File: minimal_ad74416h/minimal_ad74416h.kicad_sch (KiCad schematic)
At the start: 82 parts, among them U2 AD74416HBCPZ-RL7, U3 ADR4525BRZ

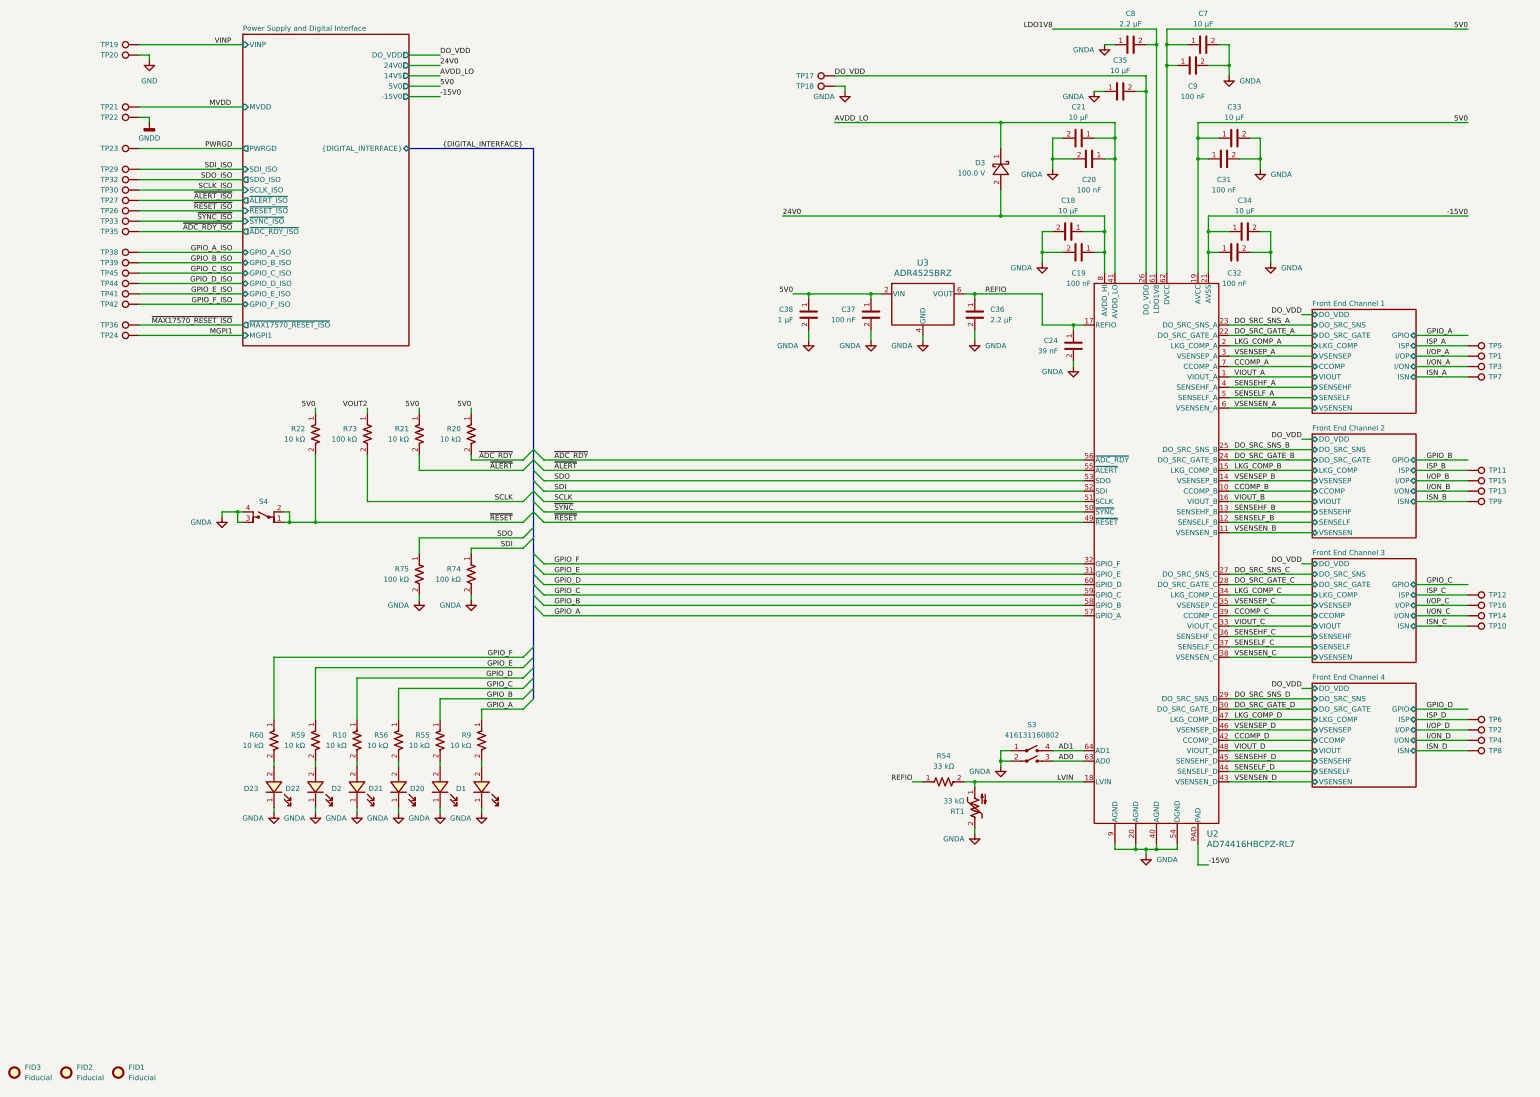
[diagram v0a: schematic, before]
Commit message: backup
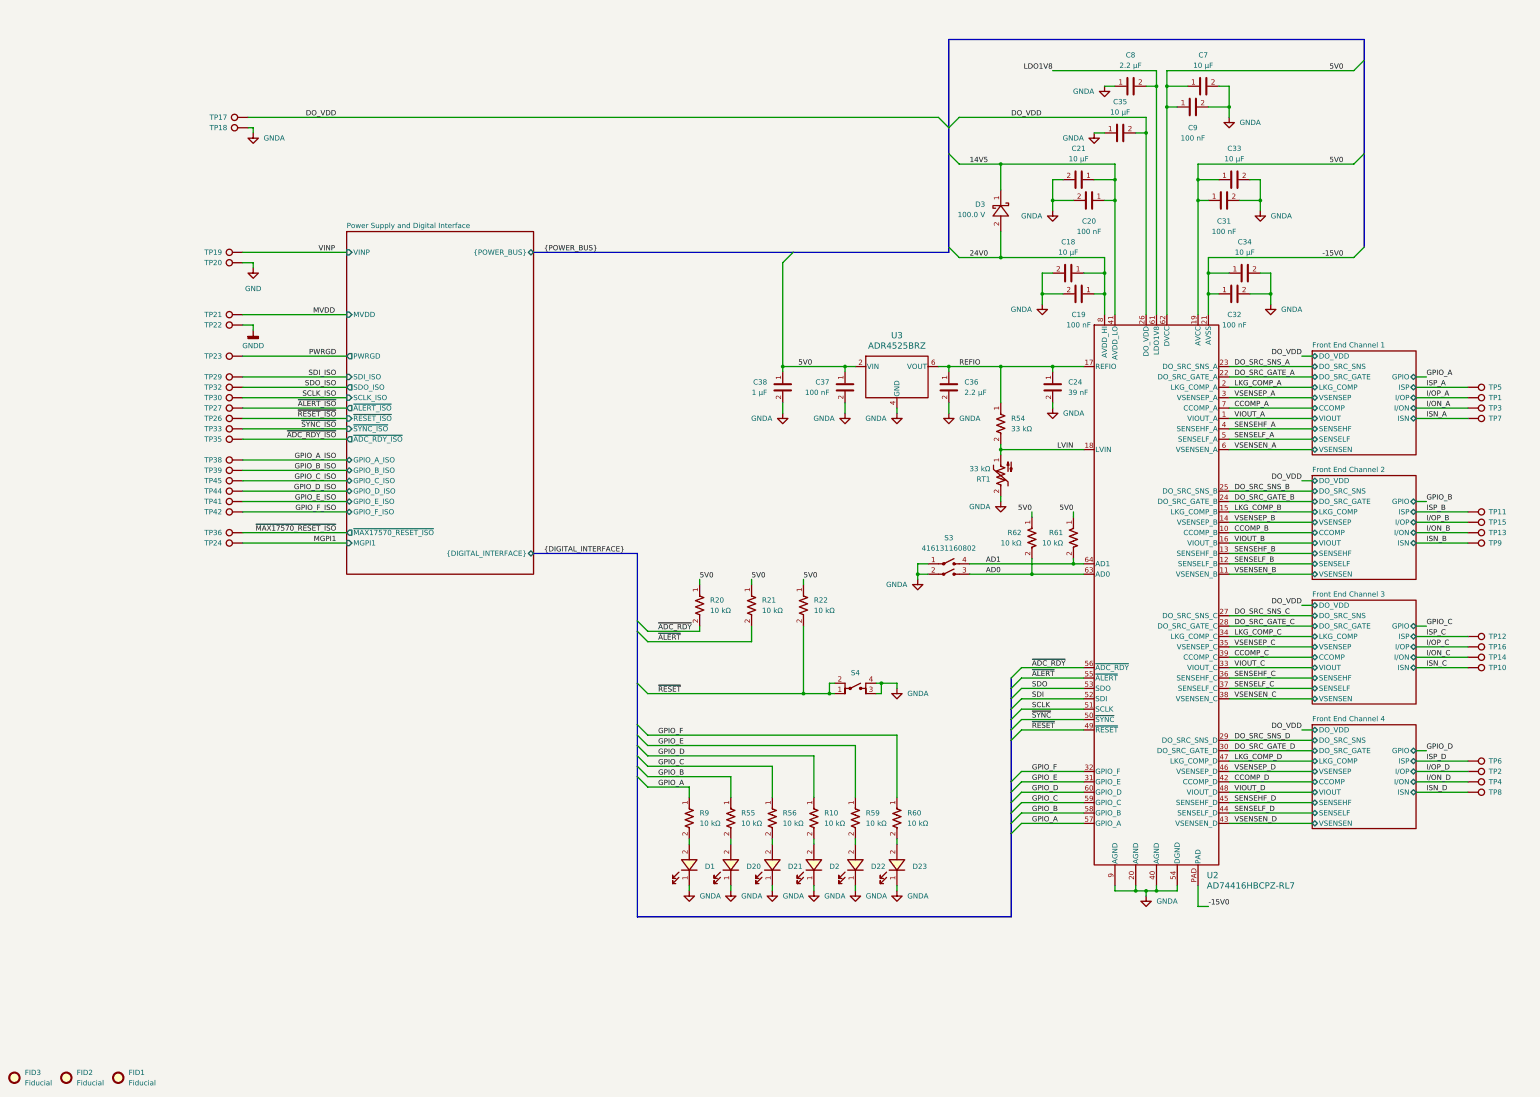
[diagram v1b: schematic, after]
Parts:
- removed R73, R74, R75: 100 kΩ, resistor_footprints:R_0402_1005Metric, symbol UNITED_RESISTORS_DATA_BASE:R_ERJ-2GEJ104X
- added R61, R62: 10 kΩ, resistor_footprints:R_0402_1005Metric, symbol UNITED_RESISTORS_DATA_BASE:R_ERJ-2RKF1002X
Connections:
- net 5V0: now also R61.1, R62.1
- net AD0: now also R62.2
- net AD1: now also R61.2
- net AVDD_LO renamed 14V5
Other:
- sheet Power Supply and Digital Interface ports: added {POWER_BUS}; removed -15V0, 14V5, 24V0, 5V0, DO_VDD
- moved on the sheet: C18, C19, C20, C21, C24, C31, C32, C33, C34, C35, C36, C37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

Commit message: backup
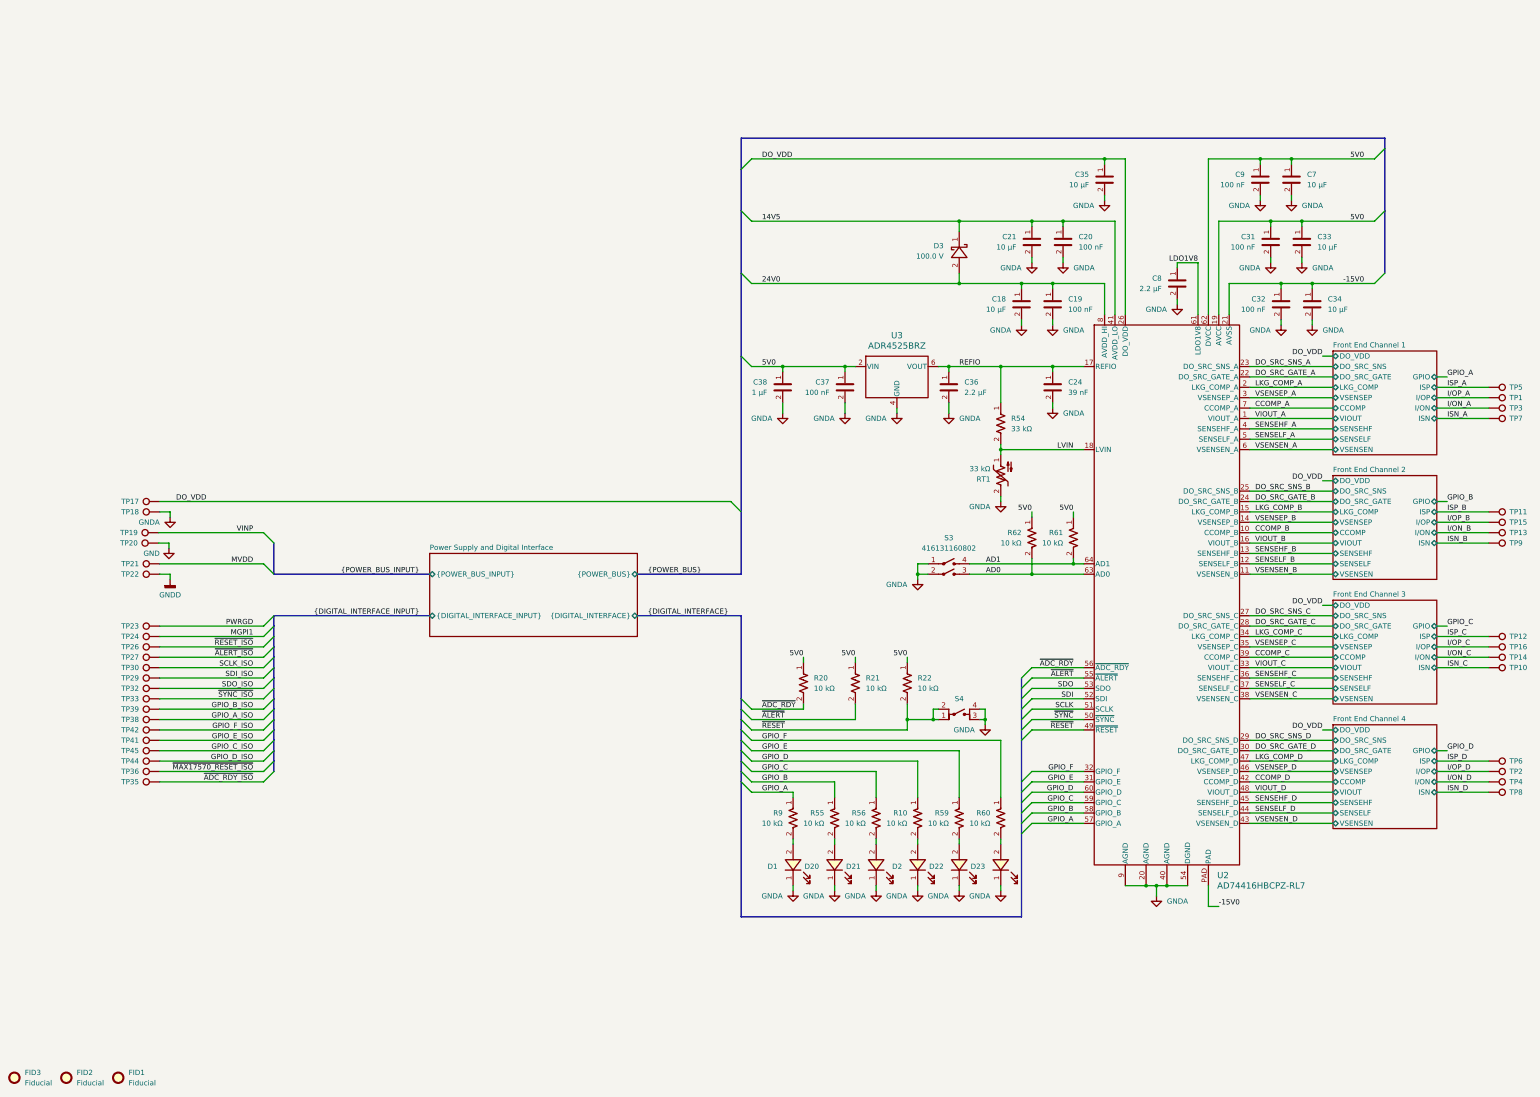
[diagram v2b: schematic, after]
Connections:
- net DO_VDD: now also C35.1; no longer C35.2
- net GNDA: now also C35.2, C8.2; no longer C35.1, C8.1
- net LDO1V8: now also C8.1; no longer C8.2
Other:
- sheet Power Supply and Digital Interface ports: added {DIGITAL_INTERFACE_INPUT}, {POWER_BUS_INPUT}; removed GPIO_A_ISO, GPIO_B_ISO, GPIO_C_ISO, GPIO_D_ISO, GPIO_E_ISO, GPIO_F_ISO, MGPI1, MVDD, PWRGD, SCLK_ISO, SDI_ISO, SDO_ISO, VINP, ~{ADC_RDY_ISO}, ~{ALERT_ISO}, ~{MAX17570_RESET_ISO}, ~{RESET_ISO}, ~{SYNC_ISO}
- moved on the sheet: C18, C19, C20, C21, C31, C32, C33, C34, C35, C7, C8, C9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
